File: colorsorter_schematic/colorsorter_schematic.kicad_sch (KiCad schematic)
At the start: 34 parts, among them J1 Conn_01x03_Pin, J2 Conn_01x03_Pin, J3 Conn_01x03_Pin, J4 Conn_01x05_Pin, J5 Conn_01x05_Pin, J6 Conn_01x03_Pin, J7 Conn_01x03_Pin, SW1 SW_SPDT, U1 PIC24FJ64GA702-I/SO, U2 ESP8266-01_ESP-01, U3 LM1117DT-3.3/NOPB, Y1 830003156B

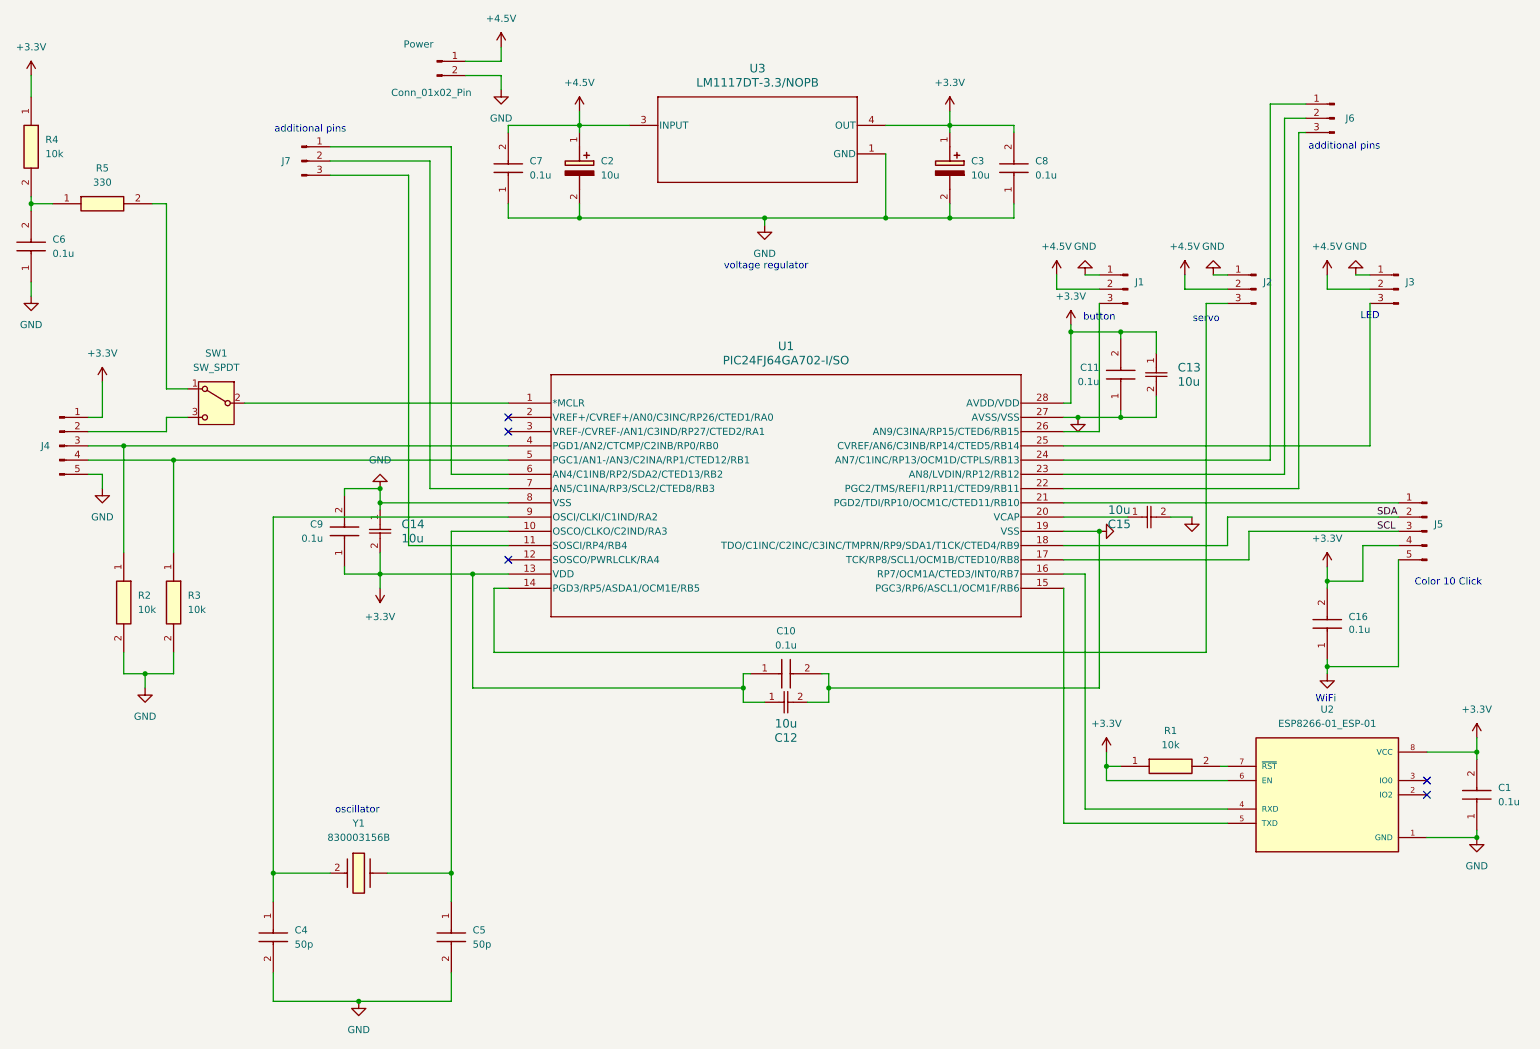
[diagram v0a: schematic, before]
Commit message: Updated schematic.
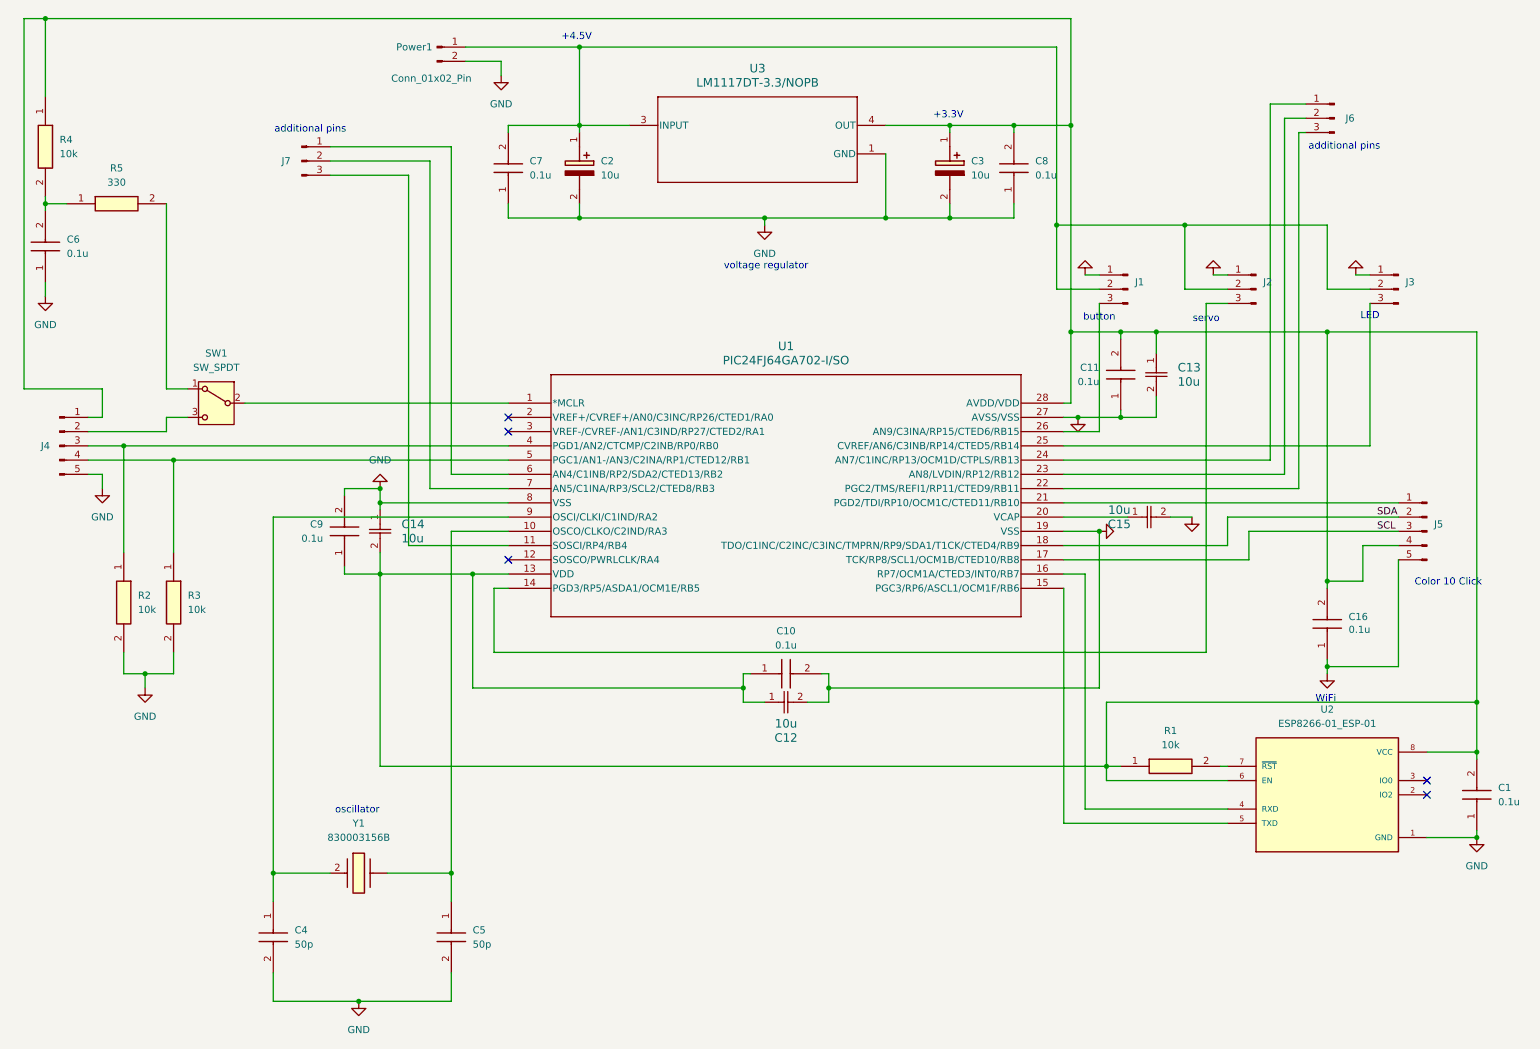
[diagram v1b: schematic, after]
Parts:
- U2: footprint ESP8266-01_ESP-01:XCVR_ESP8266-01_ESP-01 -> ESP8266-01_ESP-01:ESP8266-01_ESP-01
- renumbered Power to Power1
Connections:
- net +3.3V: no longer names the net of C1.2, C10.1, C11.2, C12.1, C13.1, C14.2, C16.2, C3.1 (+), C8.2, C9.1, J4.1 (Pin_1), J5.4 (Pin_4), R1.1, R4.1, U1.13 (VDD), U1.28 (AVDD/VDD), U2.6 (EN), U2.8 (VCC), U3.4 (OUT)
- net +4.5V: no longer names the net of C2.1 (+), C7.2, J1.2 (Pin_2), J2.2 (Pin_2), J3.2 (Pin_2), Power1.1 (Pin_1), U3.3 (INPUT)
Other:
- note added: "+3.3V"
- note added: "+4.5V"
- moved on the sheet: C6, Power1, R4, R5
